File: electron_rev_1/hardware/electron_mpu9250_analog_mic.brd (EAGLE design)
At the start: 21.2 x 46.2 mm, 33 parts, among them IC2 S25FL128SAGNFI011, IC4 MIC_I2S_SPH0645, U1 MPU-9250, U2 Value, U3 OPA322AIDBVT

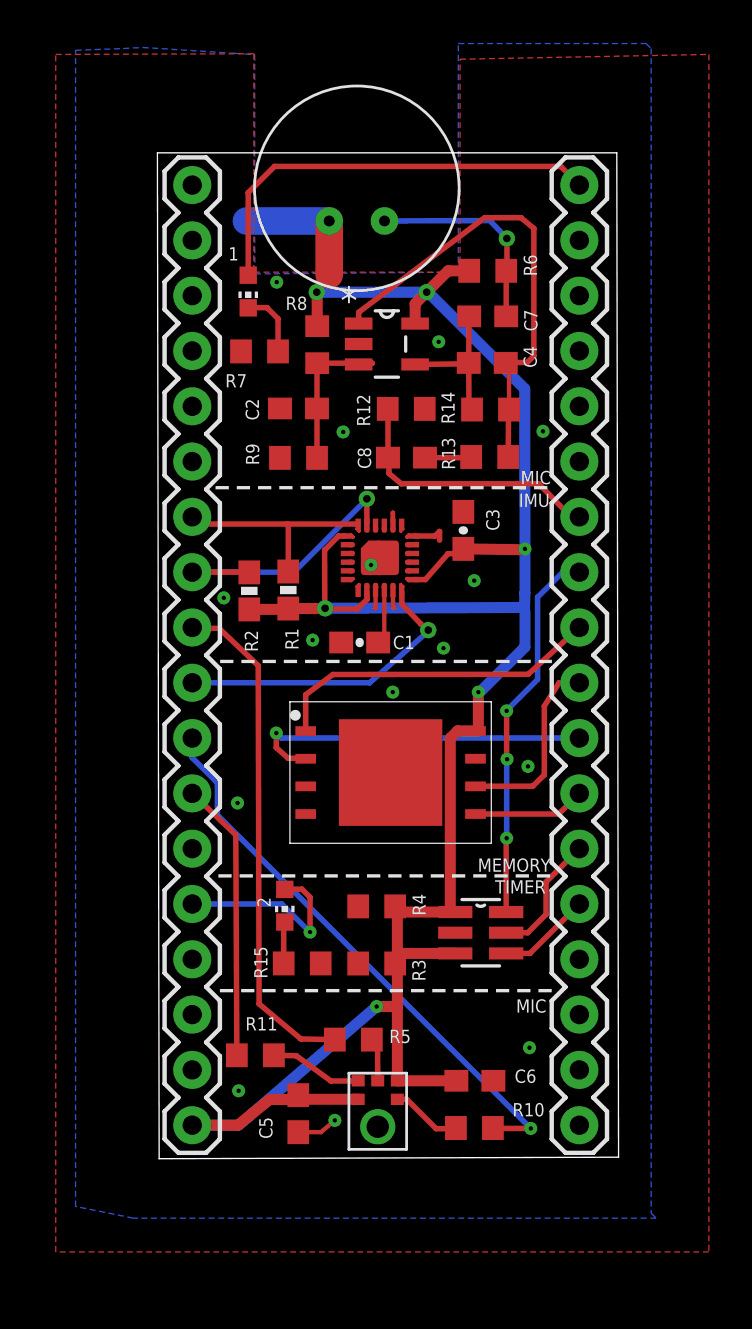
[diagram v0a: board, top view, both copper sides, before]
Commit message: cosmetic changes
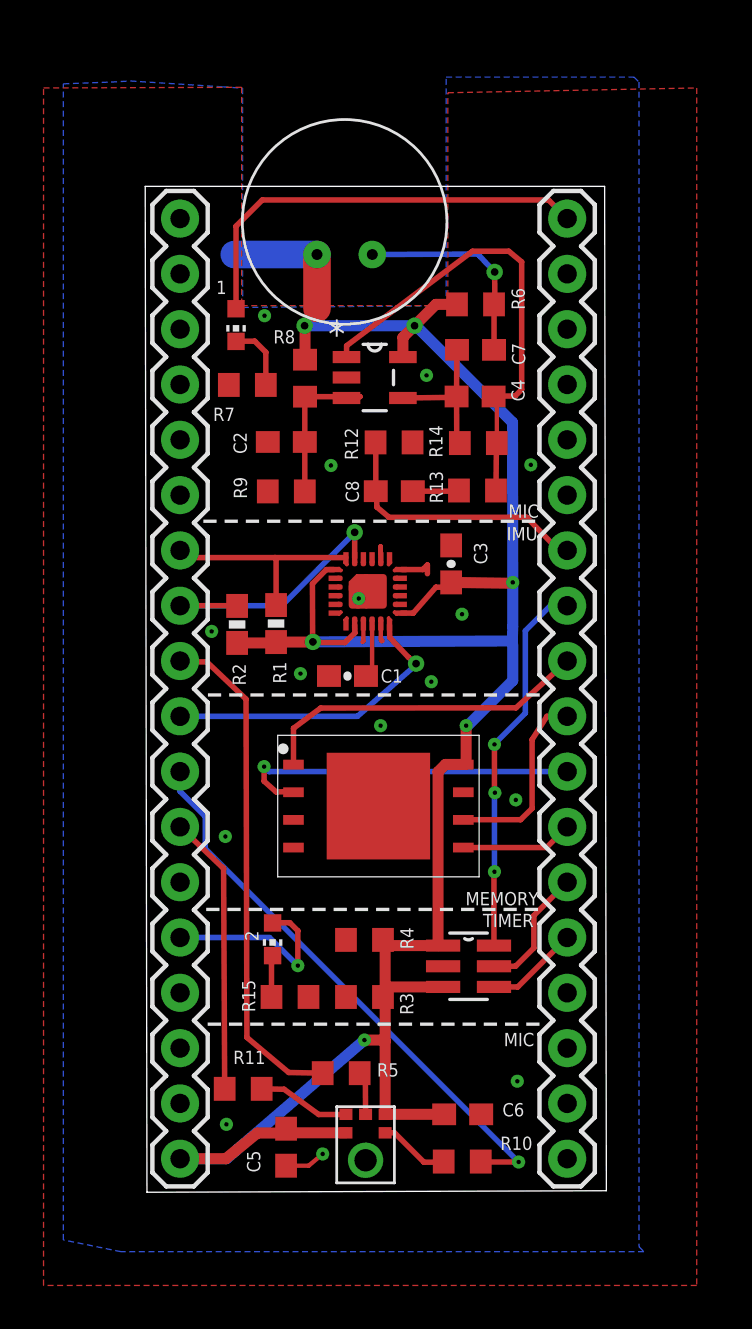
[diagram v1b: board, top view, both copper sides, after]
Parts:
- moved C8 1.64 mm to (11.4, 32.2)
- moved R1 1.64 mm to (5.95, 26.1)
- moved U1 1.64 mm to (10.2, 27.6)
- moved R15 1.64 mm to (6.59, 8.93)
- moved U2 1.64 mm to (14.8, 10.3)
- moved C6 1.64 mm to (14.5, 3.54)
- moved R10 1.64 mm to (14.5, 1.37)
- moved R5 1.64 mm to (8.94, 5.43)
- moved C5 1.64 mm to (6.41, 2.03)
- moved IC4 1.64 mm to (10.1, 2.14)
- moved R11 1.64 mm to (4.44, 4.71)
- moved C2 1.64 mm to (6.42, 34.4)
- moved C3 1.64 mm to (14.0, 28.8)
- moved C4 1.64 mm to (15.1, 36.5)
- moved C7 1.64 mm to (15.1, 38.6)
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
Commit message: passing drc
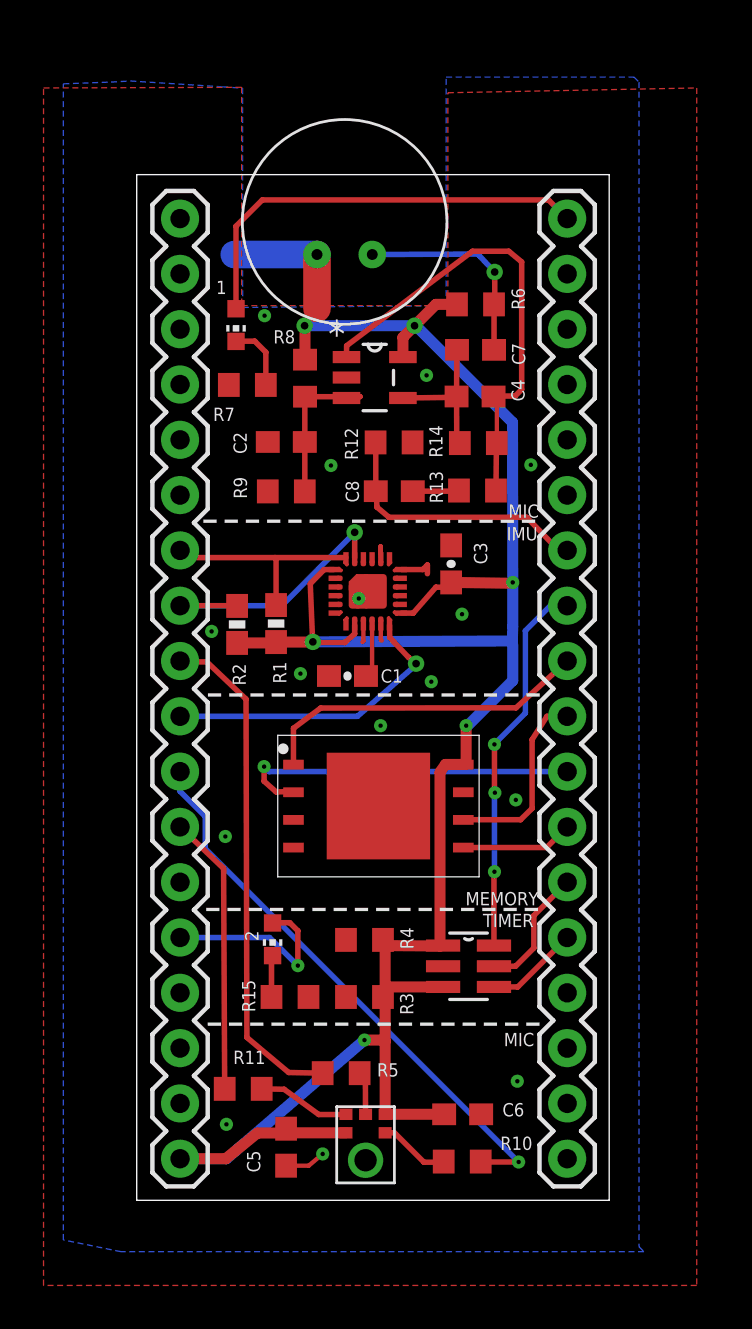
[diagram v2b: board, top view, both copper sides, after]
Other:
- board size 21.2 x 46.2 mm -> 21.7 x 47.1 mm
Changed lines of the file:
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@@
 <board>
 <plain>
-<wire x1="0.02" y1="-0.04" x2="21.12" y2="0.03" width="0" layer="20"/>
-<wire x1="21.12" y1="0.03" x2="21.04" y2="46.16" width="0" layer="20"/>
-<wire x1="21.04" y1="46.16" x2="-0.06" y2="46.16" width="0" layer="20"/>
-<wire x1="-0.06" y1="46.16" x2="0.02" y2="-0.04" width="0" layer="20"/>
+<wire x1="-0.45" y1="-0.41" x2="21.25" y2="-0.41" width="0" layer="20"/>
+<wire x1="21.25" y1="-0.41" x2="21.25" y2="46.7" width="0" layer="20"/>
+<wire x1="21.25" y1="46.7" x2="-0.45" y2="46.7" width="0" layer="20"/>
+<wire x1="-0.45" y1="46.7" x2="-0.45" y2="-0.41" width="0" layer="20"/>
 <text x="13.92" y="44.68" size="0.52" layer="26" font="vector" ratio="12">N. Klugman
 M. Podolsky</text>
@@
 <via x="2.99" y="25.72" extent="1-16" drill="0.2"/>
 <via x="9.75" y="27.23" extent="1-16" drill="0.2"/>
-<wire x1="10.805" y1="25.295" x2="10.81" y2="25.29" width="0.254" layer="1"/>
 <wire x1="9.75" y1="27.23" x2="9.83" y2="27.23" width="0.2032" layer="1"/>
 <wire x1="9.83" y1="27.23" x2="10.16" y2="27.56" width="0.2032" layer="1"/>
@@
 <wire x1="9.16" y1="2.69" x2="6.42" y2="2.69" width="0.508" layer="1"/>
 <wire x1="6.42" y1="2.69" x2="6.41" y2="2.68" width="0.2" layer="1"/>
-<wire x1="10.86" y1="11.29" x2="13.6216" y2="11.29" width="0.508" layer="1"/>
+<wire x1="10.86" y1="11.29" x2="13.48" y2="11.27" width="0.508" layer="1"/>
+<wire x1="13.48" y1="11.27" x2="13.6216" y2="11.29" width="0.508" layer="1"/>
 <wire x1="10.86" y1="11.29" x2="10.86" y2="11.55" width="0.254" layer="1"/>
 <wire x1="10.86" y1="11.55" x2="10.96" y2="11.55" width="0.254" layer="1"/>
 <wire x1="10.96" y1="11.55" x2="10.96" y2="9.02" width="0.508" layer="1"/>
-<wire x1="13.6216" y1="11.29" x2="13.39" y2="11.29" width="0.254" layer="1"/>
-<wire x1="13.39" y1="19.27" x2="13.73" y2="19.61" width="0.508" layer="1"/>
+<wire x1="13.48" y1="19.25" x2="13.73" y2="19.61" width="0.508" layer="1"/>
 <wire x1="13.73" y1="19.61" x2="14.542" y2="19.61" width="0.508" layer="1"/>
 <wire x1="14.542" y1="19.61" x2="14.55" y2="19.602" width="0.254" layer="1"/>
-<wire x1="13.39" y1="11.29" x2="13.39" y2="19.27" width="0.508" layer="1"/>
+<wire x1="13.48" y1="11.27" x2="13.48" y2="19.25" width="0.508" layer="1"/>
 <wire x1="14.75" y1="21.39" x2="16.82" y2="23.46" width="0.508" layer="16"/>
 <wire x1="14.75" y1="21.39" x2="14.68" y2="21.39" width="0.254" layer="16"/>
@@
 <wire x1="16.82" y1="25.94" x2="16.82" y2="27.97" width="0.508" layer="16"/>
 <wire x1="16.8" y1="25.18" x2="16.82" y2="25.94" width="0.508" layer="16"/>
-<wire x1="9.56" y1="26.01" x2="9.57" y2="25.65" width="0.254" layer="1"/>
-<wire x1="9.57" y1="25.65" x2="9.11" y2="25.21" width="0.254" layer="1"/>
+<wire x1="9.56" y1="26.01" x2="9.56" y2="25.61" width="0.254" layer="1"/>
+<wire x1="9.56" y1="25.61" x2="9.11" y2="25.21" width="0.254" layer="1"/>
 <wire x1="7.68" y1="25.21" x2="9.11" y2="25.21" width="0.254" layer="1"/>
 <wire x1="4.16" y1="25.19" x2="5.91" y2="25.19" width="0.508" layer="1"/>
@@
 <wire x1="7.64" y1="25.24" x2="16.8" y2="25.28" width="0.508" layer="16"/>
 <wire x1="16.8" y1="25.28" x2="16.82" y2="25.11" width="0.254" layer="16"/>
-<wire x1="8.61" y1="28.56" x2="8.26" y2="28.56" width="0.254" layer="1"/>
-<wire x1="8.26" y1="28.56" x2="7.62" y2="27.91" width="0.254" layer="1"/>
-<wire x1="7.63" y1="25.2426375" x2="7.62" y2="27.91" width="0.254" layer="1"/>
+<wire x1="8.61" y1="28.56" x2="8.16" y2="28.56" width="0.254" layer="1"/>
+<wire x1="8.16" y1="28.56" x2="7.52" y2="27.91" width="0.254" layer="1"/>
+<wire x1="7.63" y1="25.2426375" x2="7.52" y2="27.91" width="0.254" layer="1"/>
 <wire x1="7.63" y1="25.2426375" x2="7.5526375" y2="25.23" width="0.254" layer="1"/>
 <wire x1="7.6326375" y1="25.24" x2="7.64" y2="25.24" width="0.2032" layer="1"/>
@@
 </signal>
 </signals>
+<errors>
+</errors>
 </board>
 </drawing>
